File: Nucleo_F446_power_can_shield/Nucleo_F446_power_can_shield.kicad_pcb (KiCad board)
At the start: 2 copper layers, 25 parts, among them J1 ISOCAN1, J10 ISOCAN2, J11 CAN1, J12 CAN2, J13 ISOCAN1, J14 ISOCAN2, J15 CAN1, J16 CAN2, J17 RJ45, J18 RJ45, J19 I2C3, J2 ISOCAN2, J20 UART4, J3 CAN1, J4 CAN2, J5 ISOCAN1, J6 ISOCAN2, J7 CAN1, J8 CAN2, J9 ISOCAN1, M1 Isolated-Can-Transceiver-Modu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, M2 Isolated-Can-Transceiver-Modu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, M3 TJA1050_Module, M4 TJA1050_Module, U1 NUCLEO-F446RE

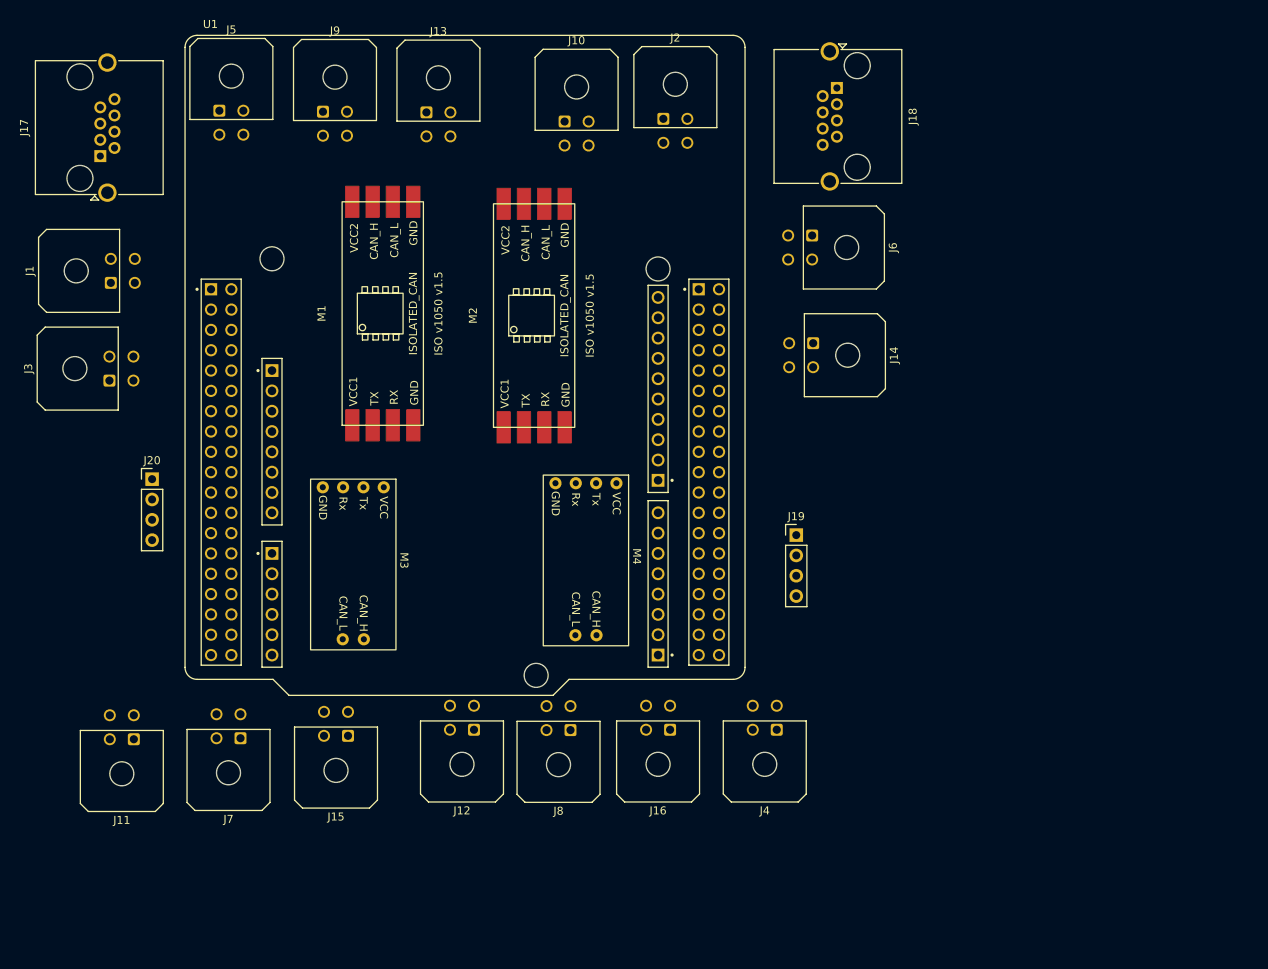
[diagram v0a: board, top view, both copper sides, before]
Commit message: shield
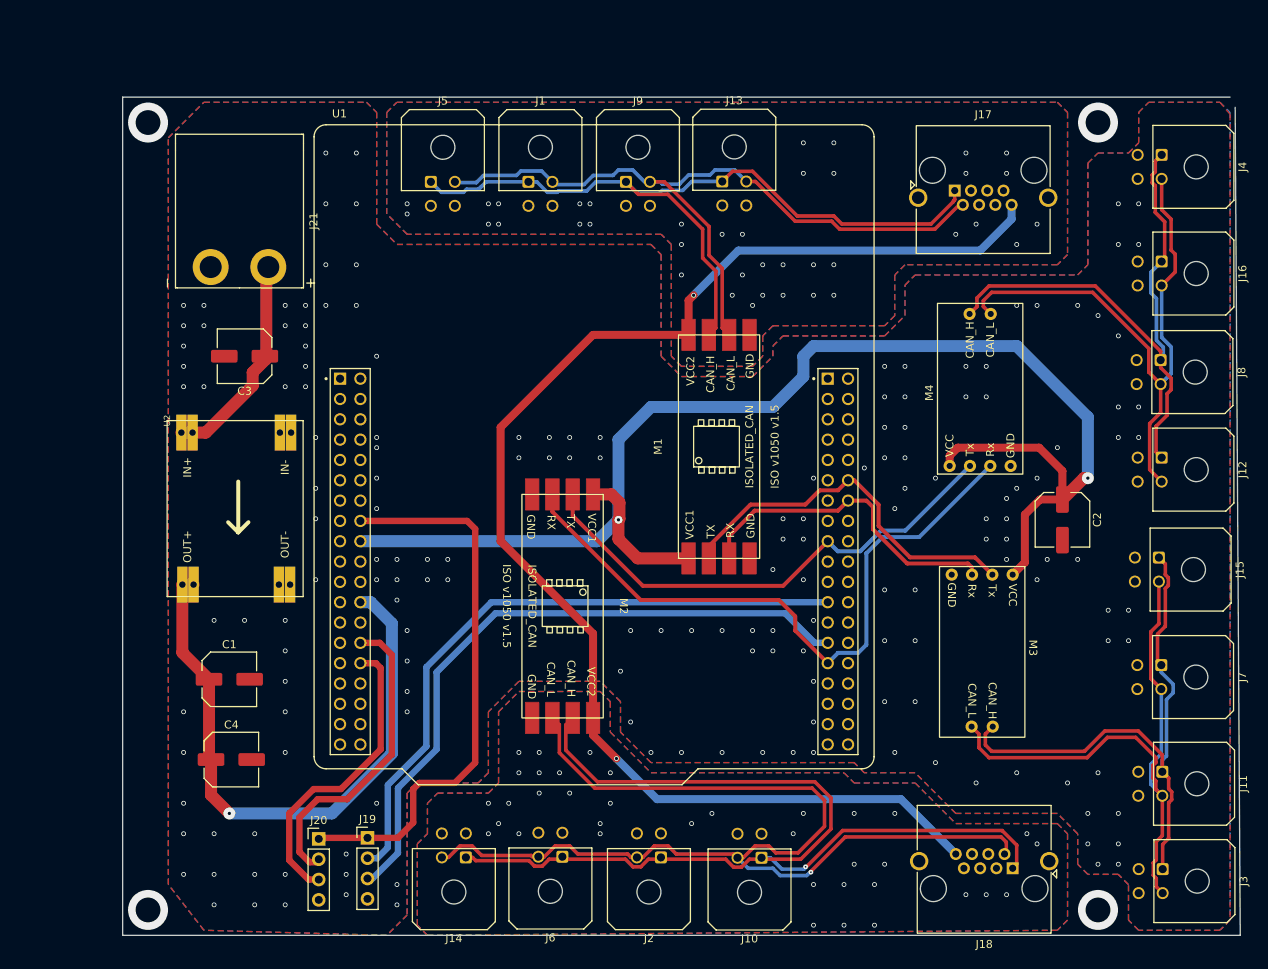
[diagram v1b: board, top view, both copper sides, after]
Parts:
- added C1: 16v220uF, Capacitor_SMD:C_Elec_6.3x7.7, F.Cu at (86.2, 104.5)
- added C2: 16v 220uF, Capacitor_SMD:C_Elec_6.3x7.7, F.Cu at (190.3, 84.6)
- added C3: 50v 47uF, Capacitor_SMD:C_Elec_6.3x7.7, F.Cu at (88.1, 64.1)
- added C4: 16v 220uF, Capacitor_SMD:C_Elec_6.3x7.7, F.Cu at (86.4, 114.5)
- added J21: xt60 male, PolyuRobotics:XT60PW-M20, F.Cu at (87.5, 47.0)
- added U2: MP1584, PolyuRobotics:DC-DC-mp1584_module, F.Cu at (78.4, 72.2)
- U1: footprint NUCLEO-F446RE:MODULE_NUCLEO-F446RE -> PolyuRobotics:NUCLEO-F446RE
- moved J3 145.1 mm to (202.9, 128.2), turned to -90 degrees
- moved J11 128.6 mm to (202.8, 116.1), turned to -90 degrees
- moved J7 115.5 mm to (202.7, 102.7), turned to -90 degrees
- moved J17 106.9 mm to (176.9, 43.4), turned to 0 degrees
- moved J15 103.8 mm to (202.4, 89.3), turned to -90 degrees
- moved J18 100.0 mm to (184.1, 128.1), turned to 180 degrees
- moved J10 95.3 mm to (152.7, 126.8), turned to 180 degrees
- moved J12 92.4 mm to (202.7, 76.8), turned to -90 degrees
- moved J2 92.3 mm to (140.1, 126.8), turned to 180 degrees
- moved J8 87.1 mm to (202.6, 64.6), turned to -90 degrees
- moved J4 86.5 mm to (202.7, 39.0), turned to -90 degrees
- moved J16 84.9 mm to (202.7, 52.3), turned to -90 degrees
- moved J6 83.7 mm to (127.8, 126.7), turned to 180 degrees
- moved M3 79.4 mm to (180.0, 100.6)
- moved J14 77.6 mm to (115.8, 126.8), turned to 180 degrees
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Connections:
- M1 pad 6: /ISO-CAN1H+ -> /ISO-CAN1+
- M1 pad 7: /ISO-CAN1H- -> /ISO-CAN1-
- U1 pad CN10_32: GND -> unconnected-(U1-PadCN10_32)
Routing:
- net +5V: track 0.00 -> 176.3 mm, vias 0 -> 2
- net <NO NET>: track 0.00 -> 173.7 mm, vias 0 -> 2
- net /ISO-CAN2-: track 0.00 -> 135.7 mm, vias 0 -> 1
- net /ISO-CAN2+: track 0.00 -> 131.9 mm, vias 0 -> 1
- net /ISO-CAN1+: track 0.00 -> 101.3 mm
- net /ISO-CAN1-: track 0.00 -> 95.8 mm
- net /PB4: track 0.00 -> 83.2 mm
- net /PB5: track 0.00 -> 82.7 mm
- net /PA8: track 0.00 -> 81.2 mm
- net VCC: track 0.00 -> 77.1 mm, vias 0 -> 1
- net /CAN1-: track 0.00 -> 75.1 mm
- net /CAN2-: track 0.00 -> 74.2 mm
- net /CAN2+: track 0.00 -> 72.5 mm
- net /CAN1+: track 0.00 -> 71.8 mm
- net +3V3: track 0.00 -> 69.9 mm
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- added copper zone on B.Cu, net GND
- added copper zone on F.Cu, net GND
- added copper zone on B.Cu, net GND1
- added copper zone on F.Cu, net GND1
- added copper zone on B.Cu, net GND2
- added copper zone on F.Cu, net GND2
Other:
- board outline added: 139.7 x 104.8 mm
